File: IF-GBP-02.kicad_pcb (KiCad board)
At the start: 2 copper layers, 65.7 x 86.3 mm, 93 parts, among them CN1 Print Motor, CN2 GB Printer Print Head, CN3 Gameboy Link Port, IC1 4A 8D1 - BGA6489, IC2 TMP87CM40AF, IC3 LH5164, IC5 TD62593A, IC6 TD62593A, IC7 458F - FMMT458TA SOT23-5, J2 Battery Connectors, Q1 B1326, Q10 BR - BCW60DR, Q11 BR - BCW60DR, Q14 24 - DTC114ECA, Q2 FR - 2SA1037, Q3 BR - BCW60DR, Q4 FR - 2SA1037, Q5 24 - DTC114ECA, Q6 BF RD - RT9169, Q7 CF RD - 2SC3650, Q8 BR - BCW60DR, Q9 FR - 2SA1037, SW1 SW_MEC_5E, SW2 SW_DPDT_x2, X1 8 MHz

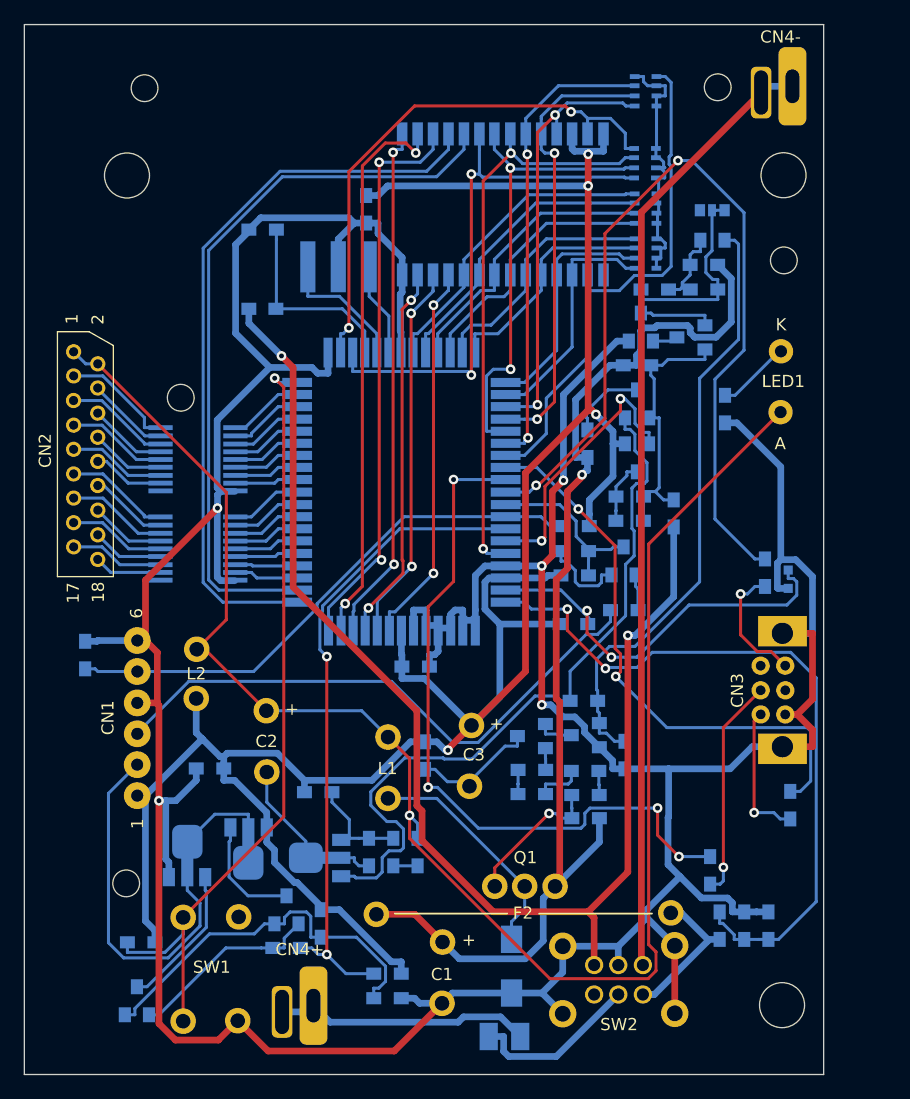
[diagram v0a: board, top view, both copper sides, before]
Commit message: Add files via upload
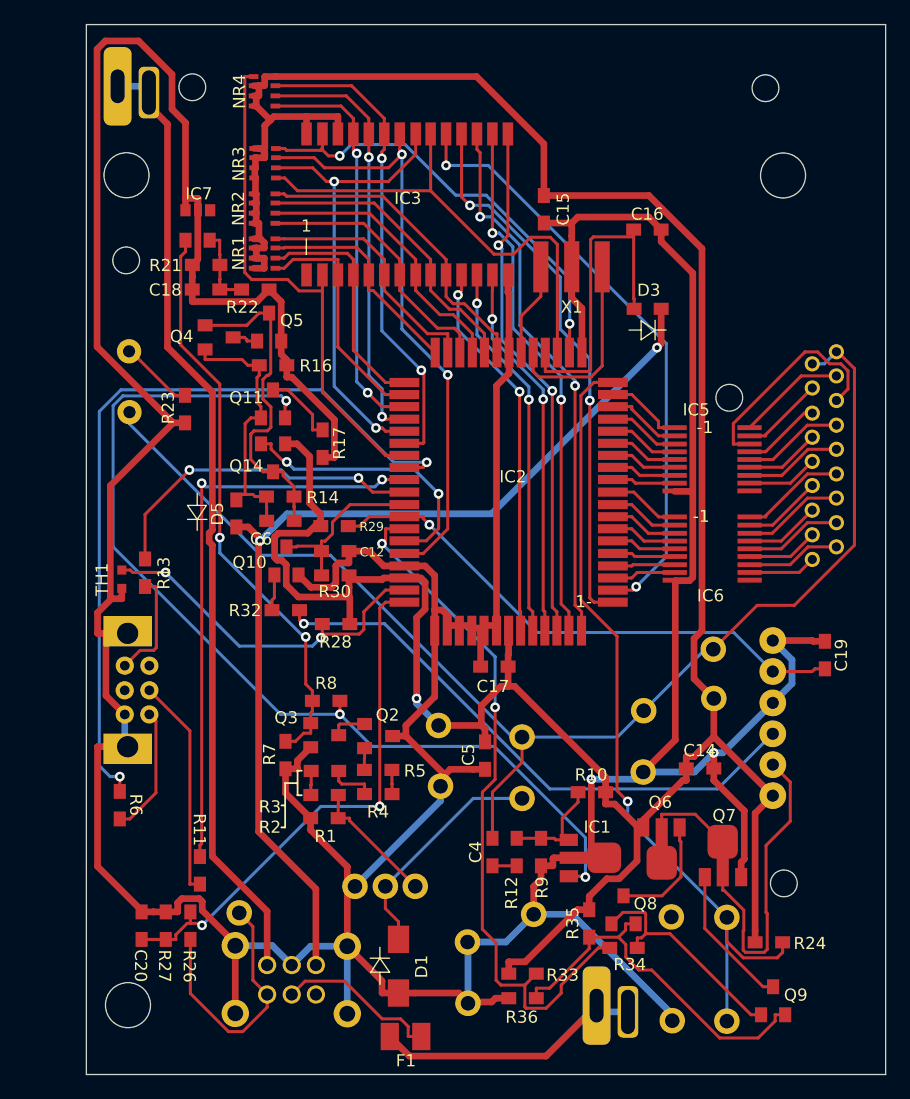
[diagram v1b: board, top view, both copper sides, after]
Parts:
- C1, C2, C3, CN1, CN2, CN3, F2, Hole1, Hole2, Hole3, Hole4, Hole5, Hole6, Hole7, Hole8, L1, L2, LED1, Q1, SW1, SW2: moved to B.Cu
- C12, C14, C15, C16, C17, C18, C19, C20, C4, C5, C6, D1, D1Diagram, D3, D3Diagram, D5, D5Diagram, F1, IC1, IC2, IC3, IC5, IC6, J2, NR1, NR2, NR3, NR4, Q10, Q11, Q14, Q2, Q3, Q5, R1, R10, R11, R12, R13, R14, R16, R17, R2, R21, R22, R23, R24, R26, R27, R28, R29, R3, R30, R32, R33, R34, R35, R36, R4, R5, R6, R7, R8, R9, TH1, X1: moved to F.Cu
- IC7: value 458F - FMMT458TA SOT23-5 -> 458F; moved to F.Cu
- Q4, Q9: value FR - 2SA1037 -> FR; moved to F.Cu
- Q6: value BF RD - RT9169 -> BF RD; moved to F.Cu
- Q7: value CF RD - 2SC3650 -> CF RD; moved to F.Cu
- Q8: value BR - BCW60DR -> BR; moved to F.Cu
- moved C19 60.6 mm to (181.1, 110.0)
- moved CN2 60.6 mm to (181.1, 93.6), turned to 180 degrees
- moved R6 55.3 mm to (123.2, 122.4)
- moved TH1 54.8 mm to (123.4, 103.8), turned to 0 degrees
- moved CN3 54.3 mm to (123.7, 112.8), turned to 180 degrees
- moved Hole5 54.1 mm to (123.8, 77.5), turned to 180 degrees
- moved Hole7 54.1 mm to (177.9, 128.8), turned to 180 degrees
- moved Hole4 54.0 mm to (123.8, 70.5), turned to 180 degrees
- moved Hole2 53.9 mm to (177.8, 70.6), turned to 180 degrees
- moved Hole6 53.8 mm to (124.0, 138.8), turned to 180 degrees
- moved LED1 53.7 mm to (124.0, 87.5), turned to 180 degrees
- moved Q9 52.3 mm to (177.0, 138.5), turned to 0 degrees
- moved CN1 52.2 mm to (176.9, 115.1), turned to 180 degrees
- moved C20 51.7 mm to (125.0, 132.3)
- moved R24 51.7 mm to (176.7, 133.7), turned to 0 degrees
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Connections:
- net /9V.F1 renamed Net-(SW2-Pad5)
- net /9V.Prefuse renamed Net-(SW2-Pad6)
- net /LED.Anode renamed Net-(L1-Pad1)
- net /LED.Cathode renamed Net-(LED1-Pad1)
- net /Route1 renamed Net-(Q1-Pad2)
- net /Route12 renamed Net-(Q7-Pad1)
- net /Route13 renamed Net-(Q8-Pad1)
- net /Route14 renamed Net-(R35-Pad1)
- net /Route15 renamed Net-(Q11-Pad2)
- net /Route16 renamed Net-(Q6-Pad1)
- net /Route19 renamed Net-(C6-Pad1)
- net /Route2 renamed Net-(R2-Pad2)
- net /Route20 renamed Net-(Q3-Pad1)
- net /Route21 renamed Net-(IC7-Pad2)
- net /Route24 renamed Net-(Q4-Pad3)
- net /Route25 renamed Net-(Q11-Pad3)
- net /Route27 renamed Net-(Q10-Pad1)
- net /Route3 renamed Net-(R2-Pad1)
- net /Route4 renamed Net-(R3-Pad2)
- net /Route5 renamed Net-(R4-Pad2)
- net /Route6 renamed Net-(R5-Pad1)
- net /Route7 renamed Net-(Q2-Pad1)
- net /Route8 renamed Net-(R12-Pad2)
- net /Route9 renamed Net-(C4-Pad1)
- C1 pad 1: /9V.Postfuse -> /GND
- C12 pad 2: /Route28 -> /GND
- C18 pad 1: /Route22 -> /GND
- C2 pad 2: /Route10 -> /GND
- C3 pad 2: /Route17 -> /GND
- C5 pad 1: /Route17 -> /GND
- C6 pad 2: /Route26 -> Net-(C6-Pad2)
- F2 pad 1: /9V.Postfuse -> /GND
- IC1 pad 2: /Route10 -> /GND
- IC7 pad 3: /Route22 -> /GND
- NR1 pad 5: /Resistor.Bus -> /VCC
- NR1 pad 6: /Resistor.Bus -> /VCC
- NR1 pad 7: /Resistor.Bus -> /VCC
- NR1 pad 8: /Resistor.Bus -> /VCC
- NR2 pad 5: /Resistor.Bus -> /VCC
- NR2 pad 6: /Resistor.Bus -> /VCC
- NR2 pad 7: /Resistor.Bus -> /VCC
- NR2 pad 8: /Resistor.Bus -> /VCC
- NR3 pad 5: /Resistor.Bus -> /VCC
- NR3 pad 6: /Resistor.Bus -> /VCC
- NR3 pad 7: /Resistor.Bus -> /VCC
- NR3 pad 8: /Resistor.Bus -> /VCC
- NR4 pad 4: /Resistor.Bus -> /VCC
- NR4 pad 6: /Resistor.Bus -> /VCC
- NR4 pad 7: /Resistor.Bus -> /VCC
- NR4 pad 8: /Resistor.Bus -> /VCC
- Q1 pad 3: /9V.Postfuse -> /GND
- Q10 pad 2: /Route28 -> /GND
- Q14 pad 3: /Route26 -> Net-(C6-Pad2)
- Q2 pad 3: /Route17 -> /GND
- Q4 pad 1: /Route23 -> Net-(C6-Pad2)
- Q5 pad 3: /Route23 -> Net-(C6-Pad2)
- R1 pad 1: /9V.Postfuse -> /GND
- R14 pad 2: /Route26 -> Net-(C6-Pad2)
- R16 pad 2: /9V.Postfuse -> /GND
- R17 pad 2: /9V.Postfuse -> /GND
- R21 pad 1: /9V.Postfuse -> /GND
- R22 pad 2: /Route22 -> /GND
- R9 pad 1: /Route10 -> /GND
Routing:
- net /GND: track 348.9 -> 453.3 mm, vias 5 -> 2
- net /9V.Postfuse: track 93.5 -> 0.00 mm, vias 1 -> 0
- net /P47: track 73.2 -> 27.2 mm
- net /VCC: track 199.8 -> 244.5 mm, vias 4 -> 1
- net Net-(L1-Pad1): track 136.9 -> 106.0 mm, vias 1 -> 0
- net Net-(C6-Pad2): track 0.00 -> 27.2 mm
- net /Resistor.Bus: track 23.2 -> 0.00 mm
- net /Off.GND: track 105.2 -> 82.0 mm
- net Net-(Q11-Pad2): track 60.3 -> 82.2 mm, vias 0 -> 3
- net /P45: track 46.8 -> 64.6 mm
- net /Route22: track 16.4 -> 0.00 mm
- net /P61: track 59.9 -> 43.9 mm
- net /D6: track 60.7 -> 45.4 mm, vias 0 -> 2
- net /Route10: track 14.0 -> 0.00 mm
- net /P46: track 59.2 -> 47.8 mm, vias 4 -> 2
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
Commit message: Add files via upload
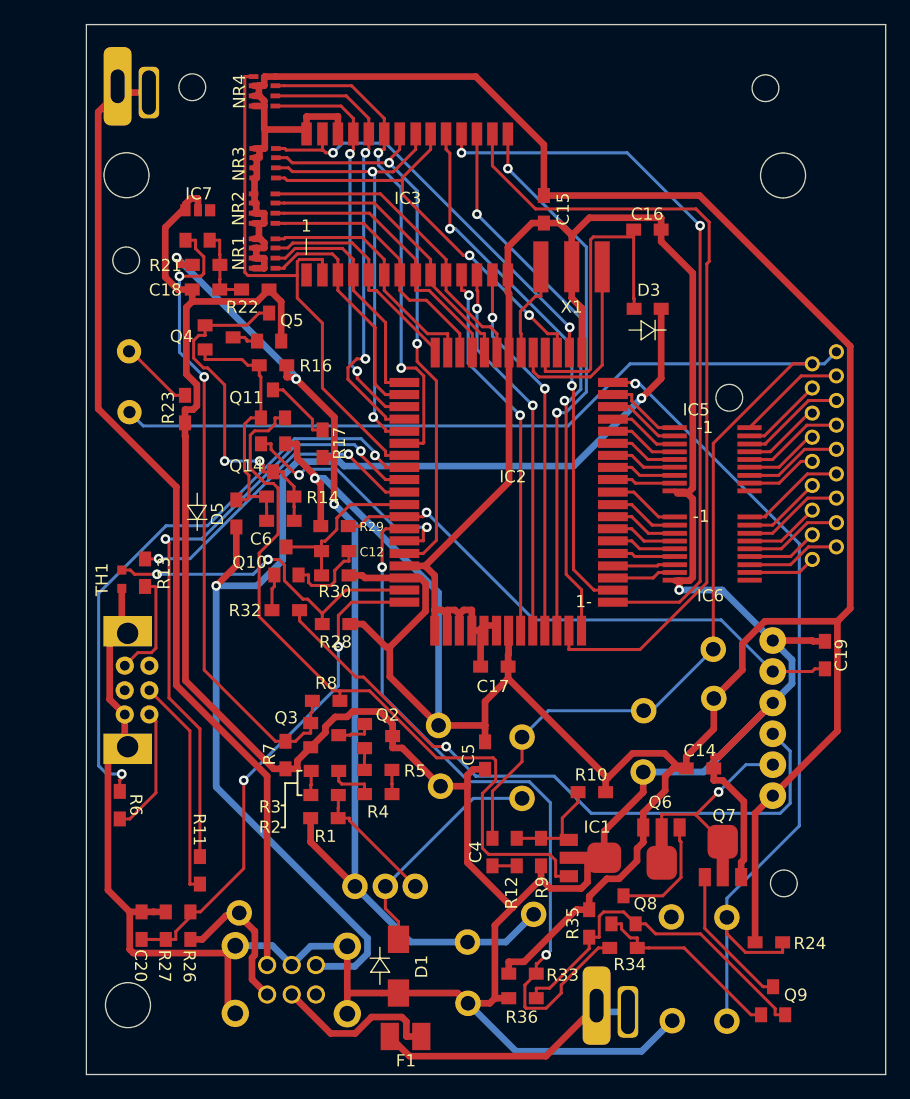
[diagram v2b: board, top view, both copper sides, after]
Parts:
- IC7: value 458F -> 458F - FMMT458TA SOT23-5
- Q4, Q9: value FR -> FR - 2SA1037
- Q6: value BF RD -> BF RD - RT9169
- Q7: value CF RD -> CF RD - 2SC3650
- Q8: value BR -> BR - BCW60DR
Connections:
- net Net-(C4-Pad1) renamed /Route9
- net Net-(C6-Pad1) renamed /Route19
- net Net-(C6-Pad2) renamed /Route23
- net Net-(IC7-Pad2) renamed /Route21
- net Net-(L1-Pad1) renamed /LED.Anode
- net Net-(LED1-Pad1) renamed /LED.Cathode
- net Net-(Q1-Pad2) renamed /Route1
- net Net-(Q10-Pad1) renamed /Route27
- net Net-(Q11-Pad2) renamed /Route15
- net Net-(Q11-Pad3) renamed /Route25
- net Net-(Q2-Pad1) renamed /Route7
- net Net-(Q3-Pad1) renamed /Route20
- net Net-(Q4-Pad3) renamed /Route24
- net Net-(Q6-Pad1) renamed /Route16
- net Net-(Q7-Pad1) renamed /Route12
- net Net-(Q8-Pad1) renamed /Route13
- net Net-(R12-Pad2) renamed /Route8
- net Net-(R2-Pad1) renamed /Route3
- net Net-(R2-Pad2) renamed /Route2
- net Net-(R3-Pad2) renamed /Route4
- net Net-(R35-Pad1) renamed /Route14
- net Net-(R4-Pad2) renamed /Route5
- net Net-(R5-Pad1) renamed /Route6
- net Net-(SW2-Pad5) renamed /9V.F1
- net Net-(SW2-Pad6) renamed /9V.Prefuse
- C1 pad 1: /GND -> /9V.Postfuse
- C12 pad 2: /GND -> /Route28
- F2 pad 1: /GND -> /9V.Postfuse
- Q1 pad 3: /GND -> /9V.Postfuse
- Q10 pad 2: /GND -> /Route28
- R1 pad 1: /GND -> /9V.Postfuse
- R16 pad 2: /GND -> /9V.Postfuse
- R17 pad 2: /GND -> /9V.Postfuse
- R21 pad 1: /GND -> /9V.Postfuse
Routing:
- net /9V.Postfuse: track 0.00 -> 87.0 mm, vias 0 -> 3
- net /GND: track 453.3 -> 394.5 mm, vias 2 -> 1
- net /VCC: track 244.5 -> 285.0 mm
- net /D4: track 43.8 -> 67.2 mm, vias 2 -> 0
- net /Route15: track 82.2 -> 62.3 mm, vias 3 -> 0
- net /CN1.P2: track 38.4 -> 20.4 mm, vias 0 -> 1
- net /Off.GND: track 82.0 -> 99.3 mm
- net /D6: track 45.4 -> 60.8 mm
- net /P45: track 64.6 -> 49.4 mm
- net /LED.Anode: track 106.0 -> 116.9 mm
- net /IC5.O3: track 18.3 -> 8.66 mm
- net /9V.Prefuse: track 21.6 -> 12.7 mm
- net /CN1.P3: track 47.3 -> 54.4 mm
- net /Route28: track 0.00 -> 7.05 mm
- net /Route20: track 47.7 -> 53.3 mm
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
